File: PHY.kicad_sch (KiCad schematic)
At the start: 52 parts, among them U1 LAN83C185-JT, Y1 25 MHz

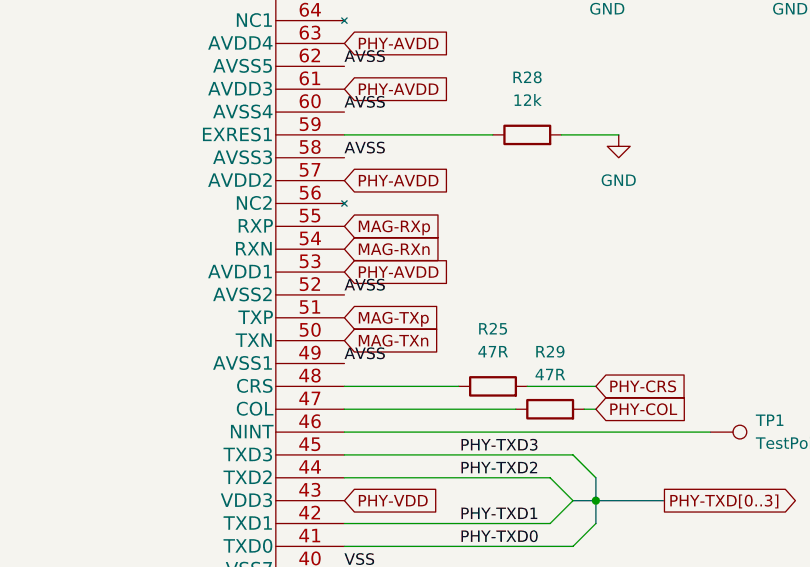
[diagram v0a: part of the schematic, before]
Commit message: did a lot more routing, phy nearly done
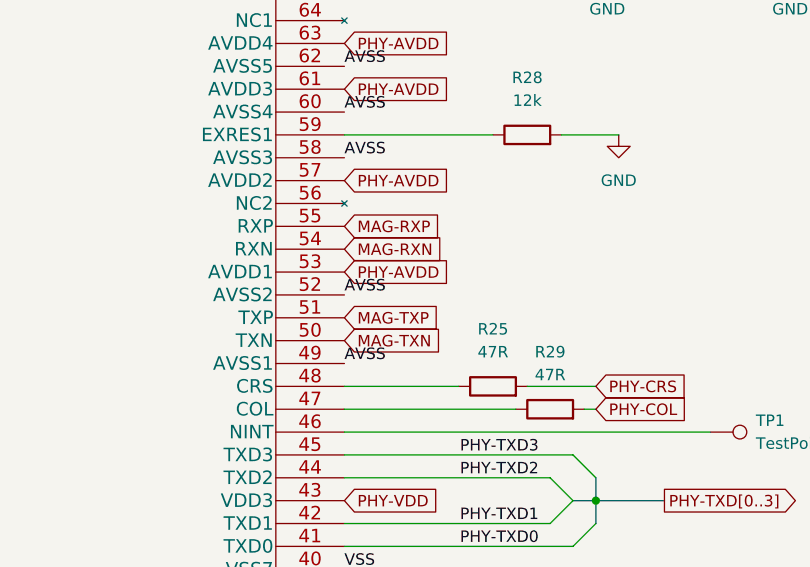
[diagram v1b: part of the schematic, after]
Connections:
- net MAG-RXn renamed MAG-RXN
- net MAG-RXp renamed MAG-RXP
- net MAG-TXn renamed MAG-TXN
- net MAG-TXp renamed MAG-TXP
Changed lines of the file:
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@@
     )
   )
-  (global_label "MAG-TXp" (shape input) (at 190.5 82.55 0) (fields_autoplaced)
+  (global_label "MAG-TXP" (shape input) (at 190.5 82.55 0) (fields_autoplaced)
     (effects (font (size 1.27 1.27)) (justify left))
-    (property "Intersheet References" "${INTERSHEET_REFS}" (id 0) (at 201.6217 82.6294 0)
+    (property "Intersheet References" "${INTERSHEET_REFS}" (id 0) (at 201.7426 82.4706 0)
       (effects (font (size 1.27 1.27)) (justify left) hide)
     )
@@
     )
   )
-  (global_label "MAG-TXn" (shape input) (at 190.5 85.09 0) (fields_autoplaced)
+  (global_label "MAG-TXN" (shape input) (at 190.5 85.09 0) (fields_autoplaced)
     (effects (font (size 1.27 1.27)) (justify left))
-    (property "Intersheet References" "${INTERSHEET_REFS}" (id 0) (at 201.6217 85.0106 0)
+    (property "Intersheet References" "${INTERSHEET_REFS}" (id 0) (at 201.8031 85.0106 0)
       (effects (font (size 1.27 1.27)) (justify left) hide)
     )
@@
     )
   )
-  (global_label "MAG-RXn" (shape input) (at 190.5 74.93 0) (fields_autoplaced)
+  (global_label "MAG-RXN" (shape input) (at 190.5 74.93 0) (fields_autoplaced)
     (effects (font (size 1.27 1.27)) (justify left))
-    (property "Intersheet References" "${INTERSHEET_REFS}" (id 0) (at 201.9241 74.8506 0)
+    (property "Intersheet References" "${INTERSHEET_REFS}" (id 0) (at 202.1055 74.8506 0)
       (effects (font (size 1.27 1.27)) (justify left) hide)
     )
@@
     )
   )
-  (global_label "MAG-RXp" (shape input) (at 190.5 72.39 0) (fields_autoplaced)
+  (global_label "MAG-RXP" (shape input) (at 190.5 72.39 0) (fields_autoplaced)
     (effects (font (size 1.27 1.27)) (justify left))
-    (property "Intersheet References" "${INTERSHEET_REFS}" (id 0) (at 201.9241 72.3106 0)
+    (property "Intersheet References" "${INTERSHEET_REFS}" (id 0) (at 202.045 72.3106 0)
       (effects (font (size 1.27 1.27)) (justify left) hide)
     )
